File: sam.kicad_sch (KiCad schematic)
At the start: 29 parts, among them IC2 74ACT244N, IC3 74ACT244N, IC4 74ACT02, IC5 74ACT138, IC6 74ACT138N, J1 JTAG, U3 XC95144XL-TQ100, U4 AS6C1008-55TIN, U5 AS6C1008-TIN, X1 14.31818MHz

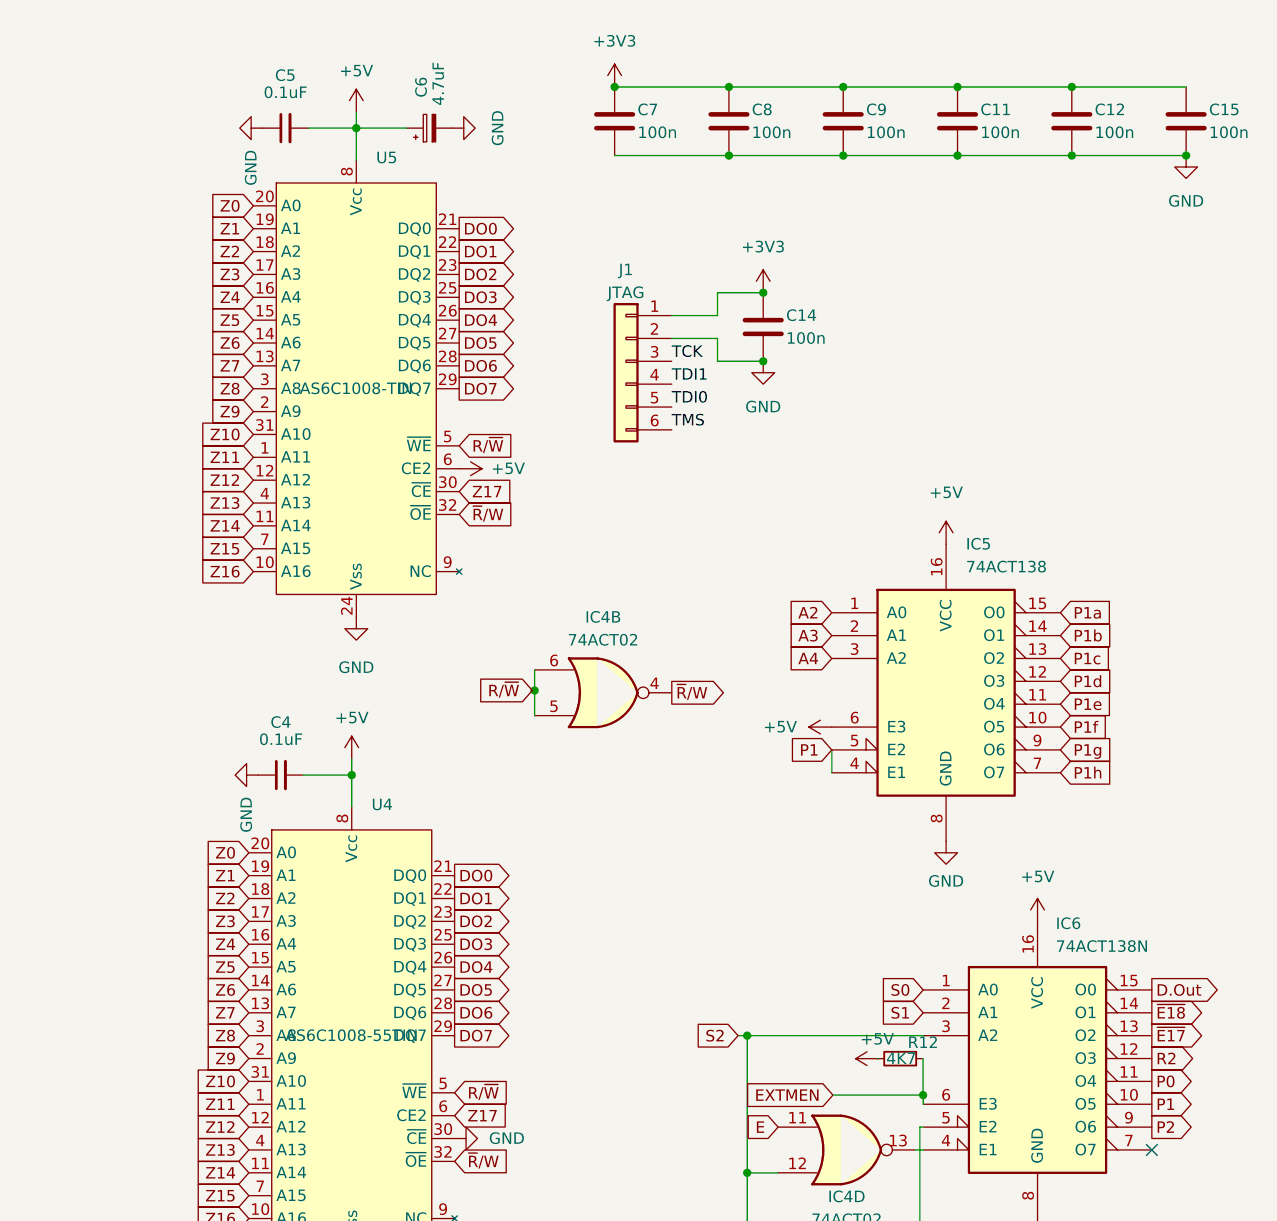
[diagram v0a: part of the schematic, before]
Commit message: Progress routing
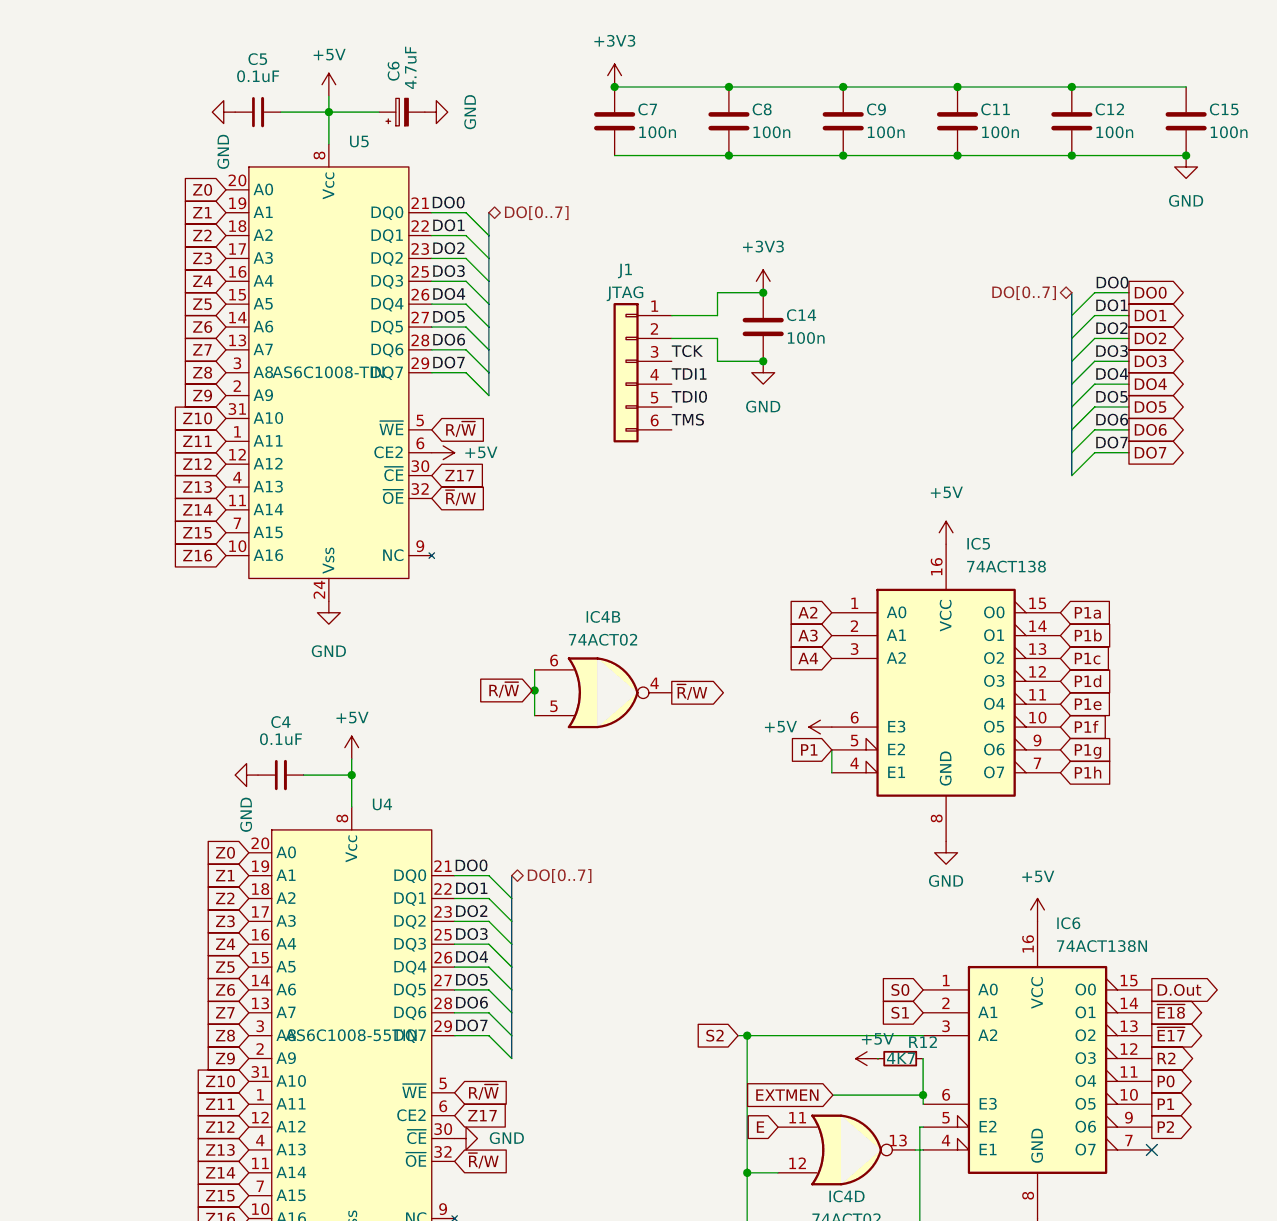
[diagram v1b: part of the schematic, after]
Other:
- moved on the sheet: C5, C6, U5
